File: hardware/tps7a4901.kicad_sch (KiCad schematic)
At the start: 9 parts, among them U8 TPS7A4901DGNR

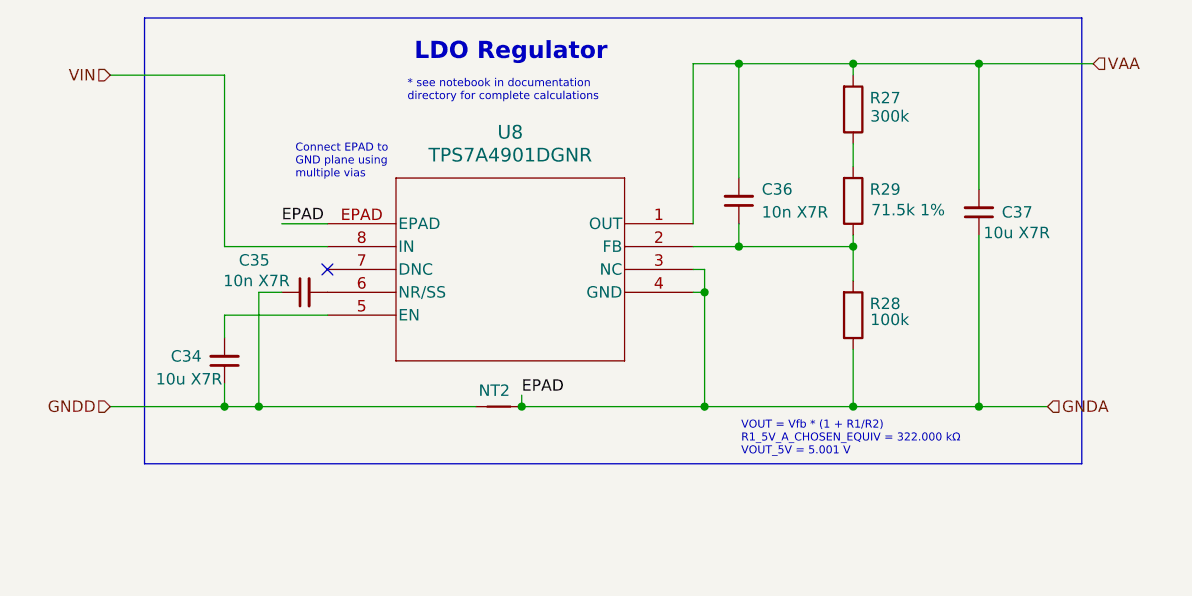
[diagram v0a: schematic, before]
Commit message: final iteration of board with proper connectors and clean layout
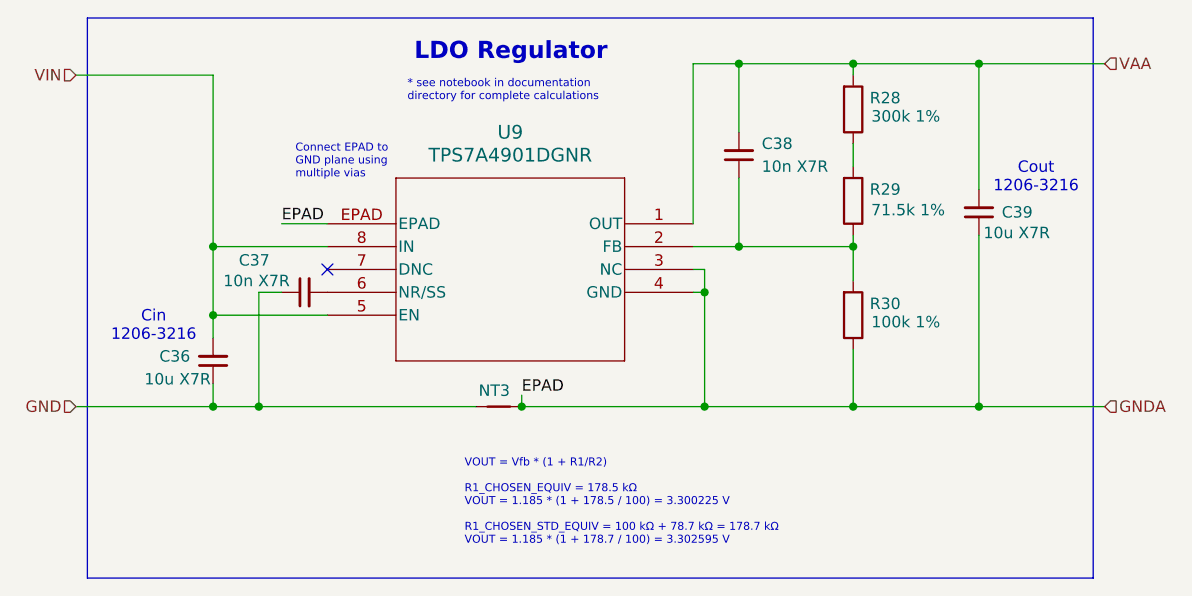
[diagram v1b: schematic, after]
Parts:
- C36: renamed from C34; footprint Capacitor_SMD:C_1206_3216Metric -> Capacitor_SMD:C_1206_3216Metric_Pad1.33x1.80mm_HandSolder
- C37: renamed from C35; footprint Capacitor_SMD:C_1206_3216Metric -> Capacitor_SMD:C_0603_1608Metric_Pad1.08x0.95mm_HandSolder
- C38: renamed from C36; footprint Capacitor_SMD:C_1206_3216Metric -> Capacitor_SMD:C_0603_1608Metric_Pad1.08x0.95mm_HandSolder
- C39: renamed from C37; footprint Capacitor_SMD:C_1206_3216Metric -> Capacitor_SMD:C_1206_3216Metric_Pad1.33x1.80mm_HandSolder
- R28: renamed from R27; value 300k -> 300k 1%; footprint (none) -> Resistor_SMD:R_0805_2012Metric_Pad1.20x1.40mm_HandSolder
- R29: footprint (none) -> Resistor_SMD:R_0805_2012Metric_Pad1.20x1.40mm_HandSolder
- R30: renamed from R28; value 100k -> 100k 1%; footprint (none) -> Resistor_SMD:R_0805_2012Metric_Pad1.20x1.40mm_HandSolder
- renumbered NT2 to NT3, U8 to U9
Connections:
- net VIN: now also C36.2, U9.5 (EN)
- net GNDD renamed GND
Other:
- note added: "Cin 1206-3216"
- note added: "Cout 1206-3216"
- note added: "VOUT = Vfb * (1 + R1/R2) R1_CHOSEN_EQUIV = 178.5 kΩ VOUT = 1.185 * (1 + 178.5 / 100) = 3.300225 V R1_CHOSEN_STD_EQUIV = 100 kΩ + 78.7 kΩ = 178.7 kΩ VOUT = 1.185 * (1 + 178.7 / 100) = 3.302595 V"
- note removed: "VOUT = Vfb * (1 + R1/R2) R1_5V_A_CHOSEN_EQUIV = 322.000 kΩ VOUT_5V = 5.001 V"
- moved on the sheet: C36, C38
